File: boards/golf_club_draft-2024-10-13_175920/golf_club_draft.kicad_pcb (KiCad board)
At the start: 2 copper layers, 1 part

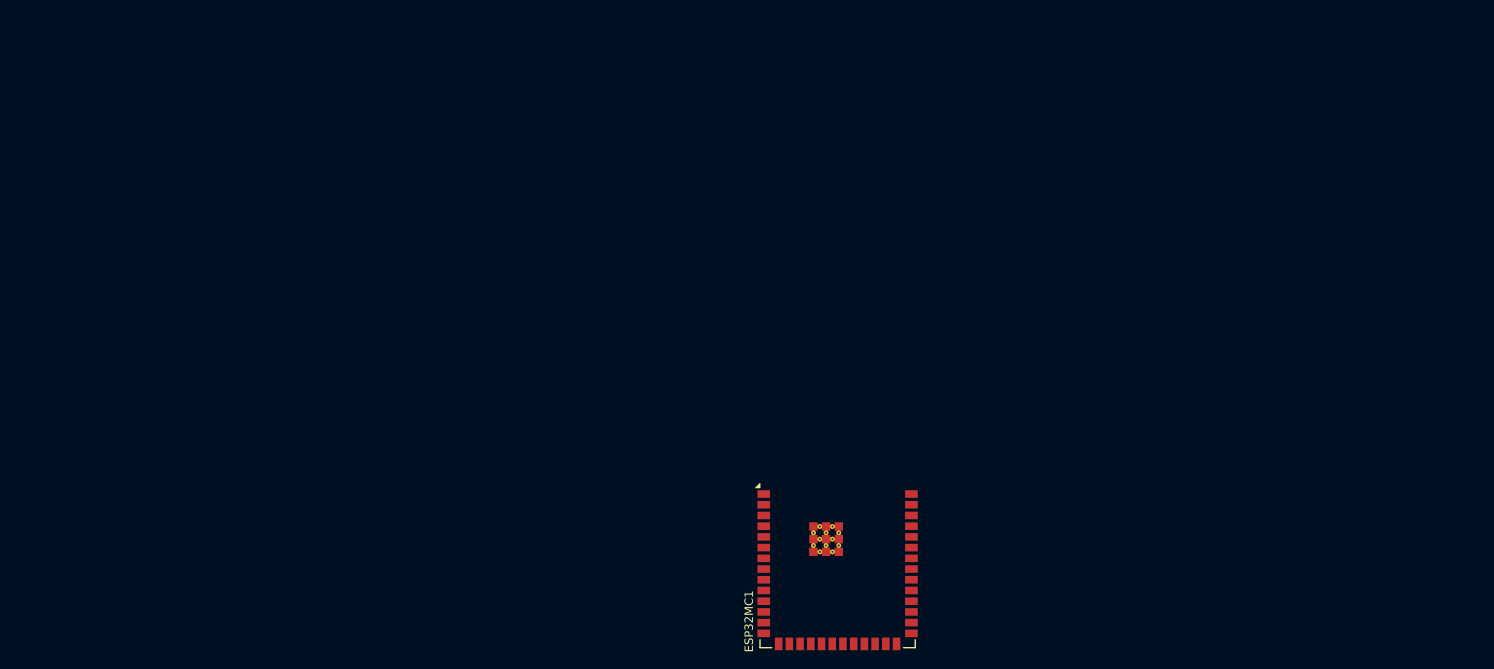
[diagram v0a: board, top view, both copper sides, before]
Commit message: Completed first draft of PCB
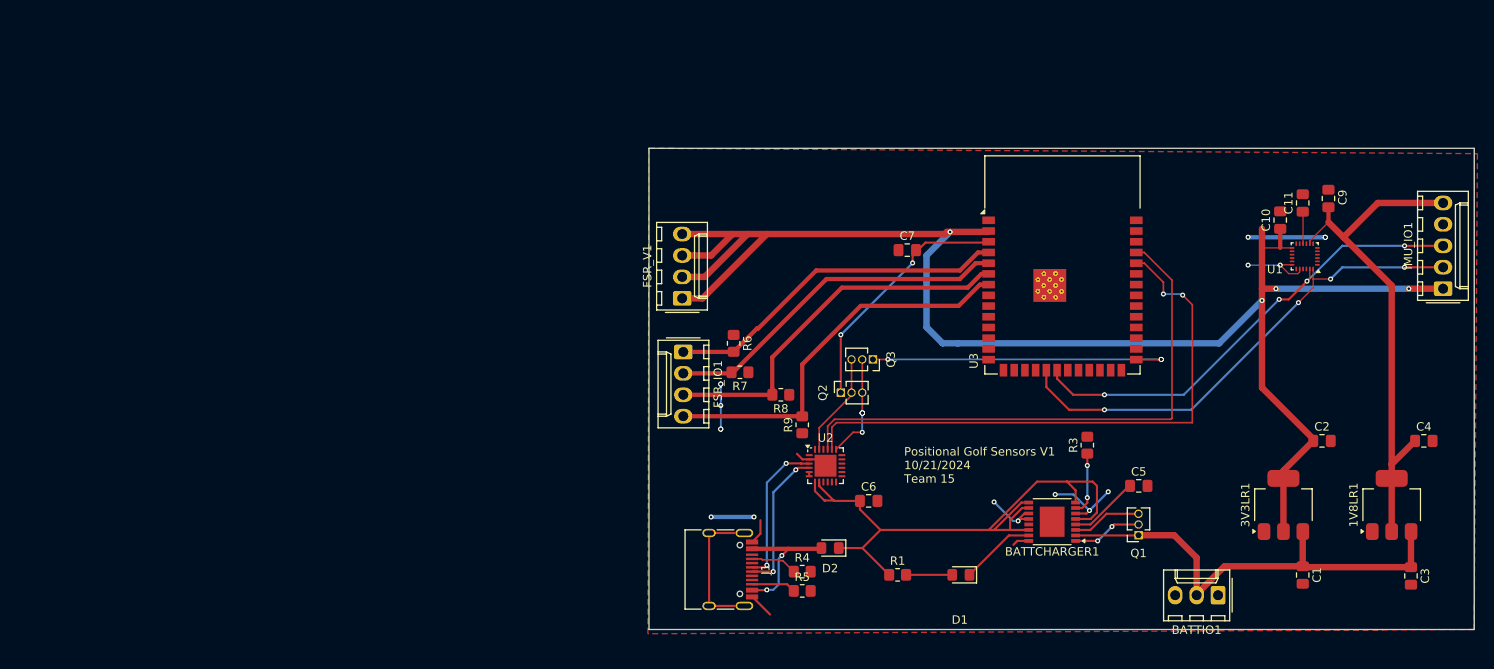
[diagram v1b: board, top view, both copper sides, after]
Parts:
- removed ESP32MC1: ESP32-S3-WROOM-2, RF_Module:ESP32-S3-WROOM-2
- added 1V8LR1: AZ1117-1.8, Package_TO_SOT_SMD:SOT-223-3_TabPin2, F.Cu at (205.1, 82.7)
- added 3V3LR1: AZ1117-3.3, Package_TO_SOT_SMD:SOT-223-3_TabPin2, F.Cu at (192.3, 82.7)
- added BATTCHARGER1: LTC4060EFE, Package_SO:TSSOP-16-1EP_4.4x5mm_P0.65mm, F.Cu at (164.9, 84.6)
- added BATTIO1: Conn_01x03_Socket, Connector_Molex:Molex_KK-254_AE-6410-03A_1x03_P2.54mm_Vertical, F.Cu at (184.5, 93.3)
- added C1: 10uF, Capacitor_SMD:C_0805_2012Metric_Pad1.18x1.45mm_HandSolder, F.Cu at (194.6, 91.0)
- added C10: 0.1uF, Capacitor_SMD:C_0805_2012Metric_Pad1.18x1.45mm_HandSolder, F.Cu at (191.9, 48.9)
- added C11: 0.1uF, Capacitor_SMD:C_0805_2012Metric_Pad1.18x1.45mm_HandSolder, F.Cu at (194.6, 46.9)
- added C2: 22uF, Capacitor_SMD:C_0805_2012Metric_Pad1.18x1.45mm_HandSolder, F.Cu at (196.8, 75.1)
- added C3: 10uF, Capacitor_SMD:C_0805_2012Metric_Pad1.18x1.45mm_HandSolder, F.Cu at (207.4, 91.1)
- added C4: 22uF, Capacitor_SMD:C_0805_2012Metric_Pad1.18x1.45mm_HandSolder, F.Cu at (208.9, 75.1)
- added C5: 1.5nF, Capacitor_SMD:C_0805_2012Metric_Pad1.18x1.45mm_HandSolder, F.Cu at (175.1, 80.4)
- added C6: 0.1uF, Capacitor_SMD:C_0805_2012Metric_Pad1.18x1.45mm_HandSolder, F.Cu at (143.1, 82.2)
- added C7: 1uF, Capacitor_SMD:C_0805_2012Metric_Pad1.18x1.45mm_HandSolder, F.Cu at (147.7, 52.5)
- added C9: 0.1uF, Capacitor_SMD:C_0805_2012Metric_Pad1.18x1.45mm_HandSolder, F.Cu at (197.6, 46.3)
- added D1: LED, LED_SMD:LED_0805_2012Metric_Pad1.15x1.40mm_HandSolder, F.Cu at (154.1, 90.9)
- added D2: D_Schottky, Diode_SMD:D_0805_2012Metric_Pad1.15x1.40mm_HandSolder, F.Cu at (138.6, 87.8)
- added FSR_IO1: Conn_01x04_Socket, Connector_Molex:Molex_KK-254_AE-6410-04A_1x04_P2.54mm_Vertical, F.Cu at (121.2, 64.5)
- added FSR_V1: Conn_01x04_Socket, Connector_Molex:Molex_KK-254_AE-6410-04A_1x04_P2.54mm_Vertical, F.Cu at (121.0, 58.2)
- added IMU_IO1: Conn_01x05_Socket, Connector_Molex:Molex_KK-254_AE-6410-05A_1x05_P2.54mm_Vertical, F.Cu at (211.2, 57.0)
- added J1: USB_C_Receptacle_USB2.0_16P, Connector_USB:USB_C_Receptacle_HRO_TYPE-C-31-M-12, F.Cu at (125.3, 90.3)
- added Q1: PNP, Connector_PinSocket_1.27mm:PinSocket_1x03_P1.27mm_Vertical, F.Cu at (175.1, 86.2)
- added Q2: NPN, Connector_PinSocket_1.27mm:PinSocket_1x03_P1.27mm_Vertical, F.Cu at (139.8, 69.3)
- added Q3: PNP, Connector_PinSocket_1.27mm:PinSocket_1x03_P1.27mm_Vertical, F.Cu at (143.6, 65.4)
- added R1: 330, Resistor_SMD:R_0805_2012Metric_Pad1.20x1.40mm_HandSolder, F.Cu at (146.6, 90.9)
- added R3: 698, Resistor_SMD:R_0805_2012Metric_Pad1.20x1.40mm_HandSolder, F.Cu at (169.0, 75.6)
- added R4: 5.1k, Resistor_SMD:R_0805_2012Metric_Pad1.20x1.40mm_HandSolder, F.Cu at (135.3, 90.6)
- added R5: 5.1k, Resistor_SMD:R_0805_2012Metric_Pad1.20x1.40mm_HandSolder, F.Cu at (135.3, 92.8)
- added R6: 10K, Resistor_SMD:R_0805_2012Metric_Pad1.20x1.40mm_HandSolder, F.Cu at (127.1, 63.5)
- added R7: 10K, Resistor_SMD:R_0805_2012Metric_Pad1.20x1.40mm_HandSolder, F.Cu at (127.9, 66.9)
- added R8: 10K, Resistor_SMD:R_0805_2012Metric_Pad1.20x1.40mm_HandSolder, F.Cu at (132.7, 69.6)
- added R9: 10K, Resistor_SMD:R_0805_2012Metric_Pad1.20x1.40mm_HandSolder, F.Cu at (135.3, 73.2)
- added U1: ICM-20948, Sensor_Motion:InvenSense_QFN-24_3x3mm_P0.4mm, F.Cu at (194.8, 53.2)
- added U2: CP2104, Package_DFN_QFN:QFN-24-1EP_4x4mm_P0.5mm_EP2.6x2.6mm, F.Cu at (138.0, 78.0)
- added U3: ESP32-S3-WROOM-1, RF_Module:ESP32-S3-WROOM-1, F.Cu at (166.1, 54.2)
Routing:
- net /3V3: track 0.00 -> 188.8 mm, vias 0 -> 4
- net /VIN: track 0.00 -> 76.0 mm
- net /RXD: track 0.00 -> 69.0 mm, vias 0 -> 2
- net /TXD: track 0.00 -> 65.9 mm
- net /1V8: track 0.00 -> 62.4 mm
- net /SDA: track 0.00 -> 58.9 mm, vias 0 -> 4
- net /SCL: track 0.00 -> 56.4 mm, vias 0 -> 4
- net GND: track 0.00 -> 56.4 mm, vias 0 -> 17
- net /VBATT: track 0.00 -> 55.2 mm
- net /FSR4: track 0.00 -> 46.3 mm
- net /FSR3: track 0.00 -> 44.7 mm
- net /FSR2: track 0.00 -> 41.6 mm
- net /FSR1: track 0.00 -> 41.1 mm
- net /GPIO0: track 0.00 -> 37.1 mm, vias 0 -> 3
- net /RESET: track 0.00 -> 29.5 mm, vias 0 -> 2
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- added copper zone on F.Cu, net GND
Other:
- board outline added: 97.8 x 57 mm
- board text added: "Positional Golf Sensors V1 10/21/2024 Team 15"

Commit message: 3rd round PCB order revisions
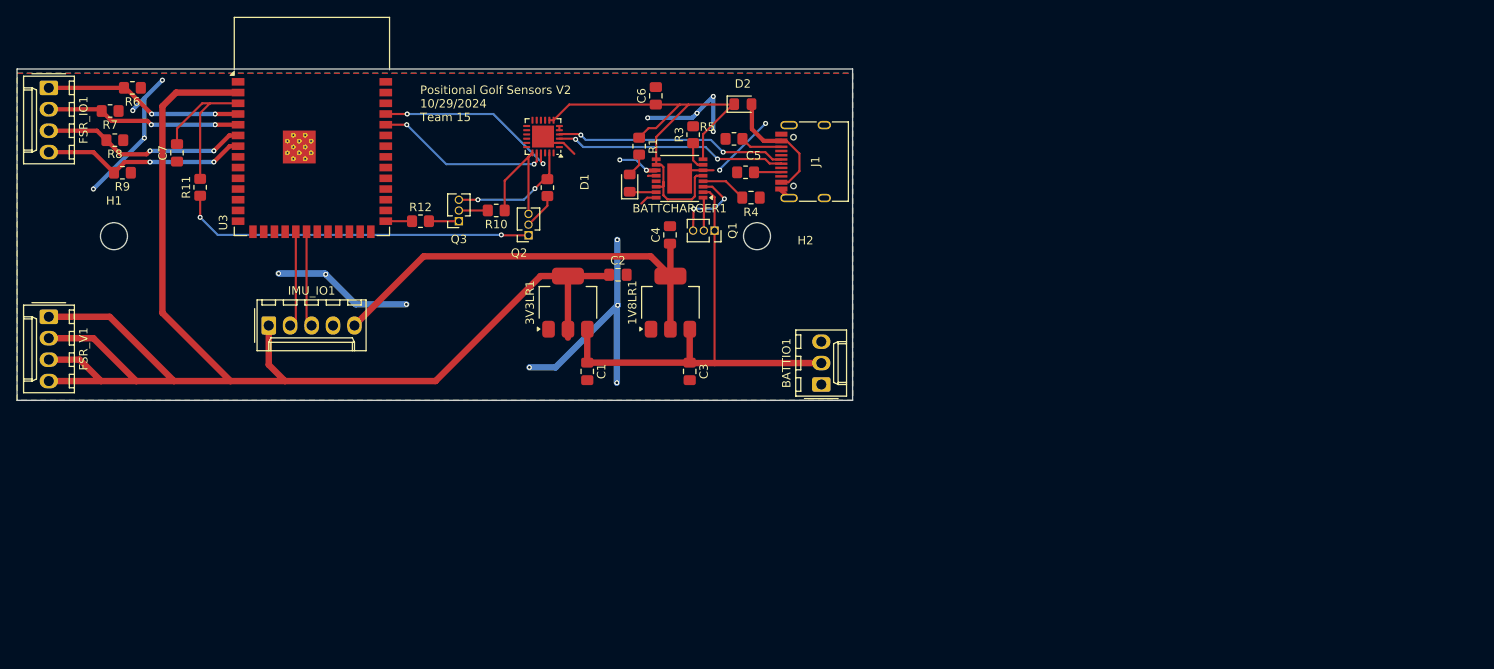
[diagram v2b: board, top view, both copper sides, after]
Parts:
- removed C10, C11, C9: 0.1uF, Capacitor_SMD:C_0805_2012Metric_Pad1.18x1.45mm_HandSolder
- removed U1: ICM-20948, Sensor_Motion:InvenSense_QFN-24_3x3mm_P0.4mm
- added H1: MountingHole, MountingHole:MountingHole_3.2mm_M3, F.Cu at (53.7, 50.8)
- added H2: MountingHole, MountingHole:MountingHole_3.2mm_M3, F.Cu at (129.9, 50.8)
- added R10: 10K, Resistor_SMD:R_0805_2012Metric_Pad1.20x1.40mm_HandSolder, F.Cu at (99.0, 47.8)
- added R11: 10K, Resistor_SMD:R_0805_2012Metric_Pad1.20x1.40mm_HandSolder, F.Cu at (63.9, 45.0)
- added R12: 10K, Resistor_SMD:R_0805_2012Metric_Pad1.20x1.40mm_HandSolder, F.Cu at (90.0, 49.0)
- added R2: 10K, Resistor_SMD:R_0805_2012Metric_Pad1.20x1.40mm_HandSolder, F.Cu at (105.1, 45.0)
- moved IMU_IO1 139.2 mm to (72.0, 61.4), turned to 0 degrees
- moved C4 92.6 mm to (119.6, 50.6), turned to 90 degrees
- moved U3 90.4 mm to (77.2, 37.8)
- moved C3 88.8 mm to (121.9, 66.8)
- moved 1V8LR1 88.8 mm to (119.6, 58.7)
- moved C1 88.2 mm to (109.8, 66.8)
- moved 3V3LR1 88.1 mm to (107.5, 58.7)
- moved C7 87.3 mm to (61.2, 40.9), turned to 90 degrees
- moved R9 85.9 mm to (54.7, 43.3), turned to 180 degrees
- moved C2 85.7 mm to (113.4, 55.4)
- moved R8 84.5 mm to (53.8, 39.4)
- moved FSR_IO1 81.4 mm to (46.0, 33.2)
- moved R7 80.8 mm to (53.2, 36.0)
- moved R6 77.4 mm to (55.9, 33.2), turned to 180 degrees
- moved FSR_V1 75.1 mm to (46.0, 60.4), turned to -90 degrees
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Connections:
- J1 pad S1: unconnected-(J1-SHIELD-PadS1) -> GND
- Q2 pad 1: /RESET -> Net-(Q2-C)
- Q2 pad 2: /DTR -> Net-(Q2-B)
- Q3 pad 1: /GPIO0 -> Net-(Q3-C)
- Q3 pad 2: /RTS -> Net-(Q3-B)
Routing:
- net /RXD: track 69.0 -> 21.0 mm
- net /SDA: track 58.9 -> 11.4 mm, vias 4 -> 0
- net GND: track 56.4 -> 103.7 mm, vias 17 -> 19
- net /SCL: track 56.4 -> 11.4 mm, vias 4 -> 0
- net /TXD: track 65.9 -> 22.5 mm, vias 0 -> 2
- net Net-(Q2-C): track 0.00 -> 42.3 mm, vias 0 -> 2
- net /GPIO0: track 37.1 -> 3.11 mm, vias 3 -> 0
- net /FSR4: track 46.3 -> 24.7 mm, vias 0 -> 2
- net /FSR3: track 44.7 -> 24.6 mm, vias 0 -> 2
- net /3V3: track 188.8 -> 169.6 mm, vias 4 -> 0
- net /FSR2: track 41.6 -> 23.2 mm, vias 0 -> 2
- net /FSR1: track 41.1 -> 23.7 mm, vias 0 -> 2
- net unconnected-(J1-SHIELD-PadS1): track 17.0 -> 0.00 mm
- net /VIN: track 76.0 -> 59.0 mm
- net /1V8: track 62.4 -> 52.0 mm
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- added copper zone on B.Cu, net GND
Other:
- board size 97.8 x 57 mm -> 99 x 39.3 mm
- board text added: "Positional Golf Sensors V2 10/29/2024 Team 15"
- board text removed: "Positional Golf Sensors V1 10/21/2024 Team 15"
